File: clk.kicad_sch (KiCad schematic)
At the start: 30 parts, among them U46 SY75602BTWL-TR, U7 SY75602BTWL-TR, U8 SI5338B-B-GM, U9 LMK1C1102DQFT

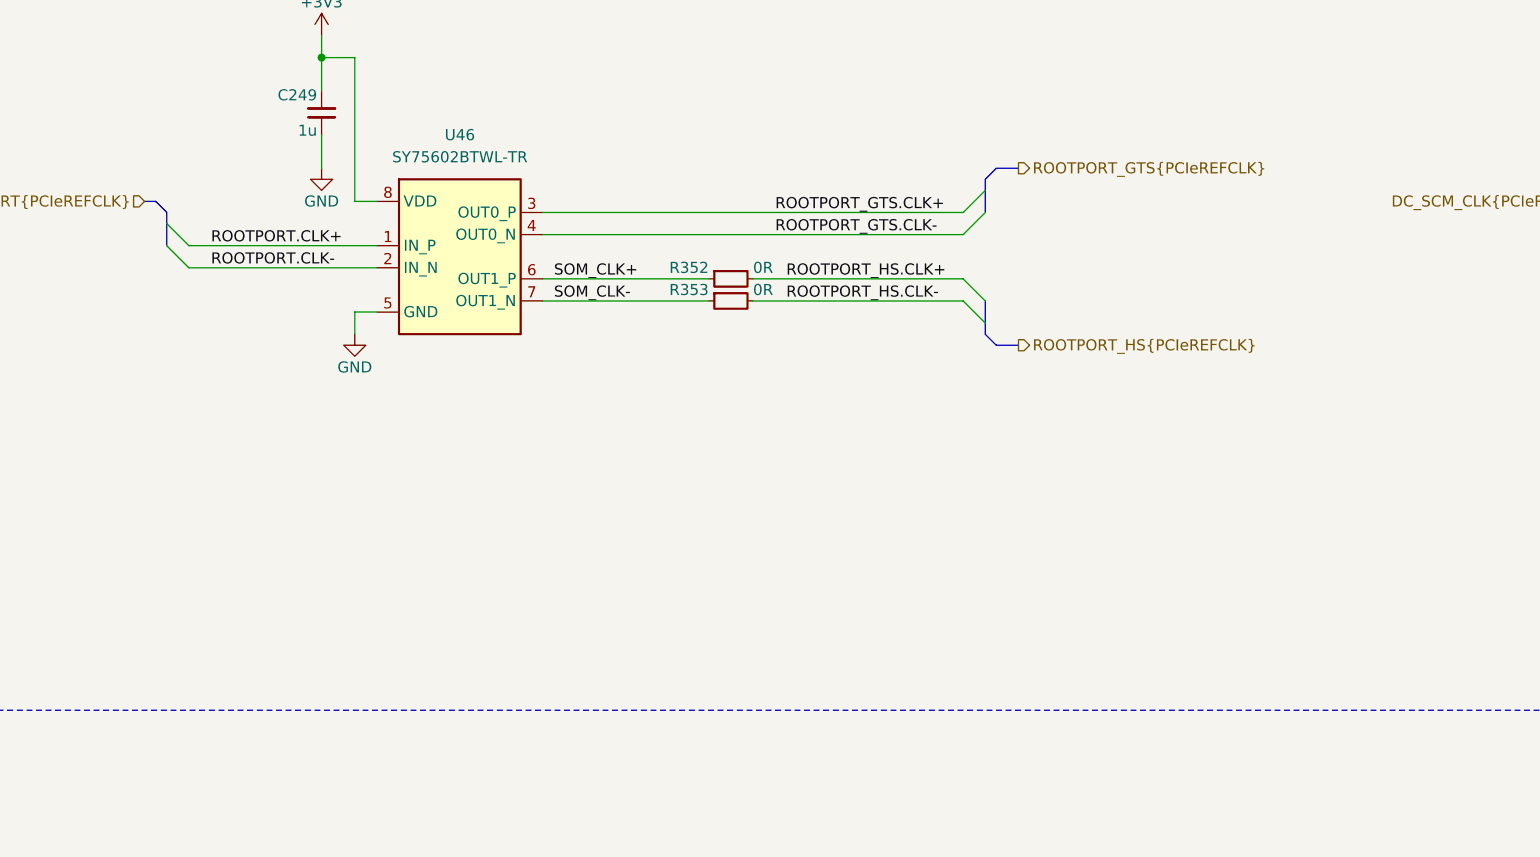
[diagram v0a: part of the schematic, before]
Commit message: [#100687] Add clocks
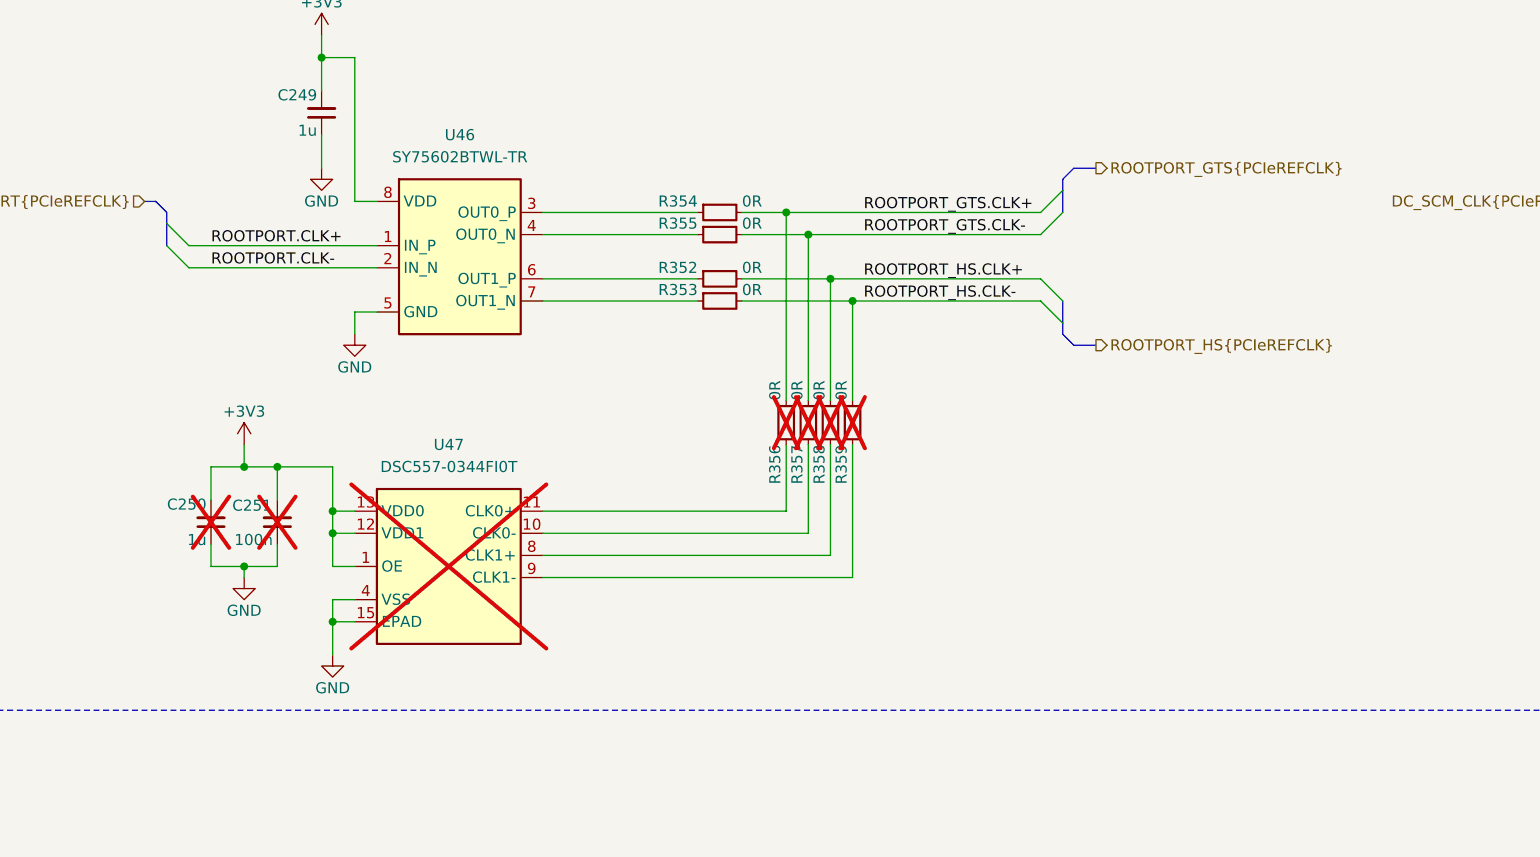
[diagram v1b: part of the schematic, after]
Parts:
- added C250: C_1u_25V_0402, antmicro-footprints:C_0402_1005Metric, symbol antmicroCapacitors0402:C_1u_25V_0402
- added C251: C_100n_0402, antmicro-footprints:C_0402_1005Metric, symbol antmicroCapacitors0402:C_100n_0402
- added R354, R355, R356, R357, R358, R359: R_0R_0402, antmicro-footprints:R_0402_1005Metric, symbol antmicroResistors0402:R_0R_0402
- added U47: DSC557-0344FI0T, antmicro-footprints:VQFN-14-1EP_3.2x2.5mm_P0.5mm_Layout4x3, symbol antmicroClockTimingRealTimeClocks:DSC557-0344FI0T
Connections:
- net +3V3: now also C250.2, C251.2, U47.1 (OE), U47.12 (VDD1), U47.13 (VDD0)
- net GND: now also C250.1, C251.1, U47.15 (EPAD), U47.4 (VSS)
- net ROOTPORT_GTS.CLK+: now also R354.2, R356.2; no longer U46.3 (OUT0_P)
- net ROOTPORT_GTS.CLK-: now also R355.2, R357.2; no longer U46.4 (OUT0_N)
- net ROOTPORT_HS.CLK+: now also R358.2
- net ROOTPORT_HS.CLK-: now also R359.2
- net SOM_CLK+: no longer R352.1, U46.6 (OUT1_P)
- net SOM_CLK-: no longer R353.1, U46.7 (OUT1_N)
- new net: R356.1, U47.11 (CLK0+)
- new net: R354.1, U46.3 (OUT0_P)
- new net: R352.1, U46.6 (OUT1_P)
- new net: R359.1, U47.9 (CLK1-)
- new net: R357.1, U47.10 (CLK0-)
- new net: U47.14 (NC), U47.2 (NC), U47.3 (NC), U47.5 (NC), U47.6 (NC), U47.7 (NC)
- new net: R358.1, U47.8 (CLK1+)
- new net: R355.1, U46.4 (OUT0_N)
- new net: R353.1, U46.7 (OUT1_N)
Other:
- moved on the sheet: R352, R353
